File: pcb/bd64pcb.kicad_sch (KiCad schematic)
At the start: 225 parts, among them J1 USB_C_Receptacle_USB2.0, SW1 SW_Push, U1 ATmega32U4-MU, U2 IS31FL3733-QF, Y1 16MHz

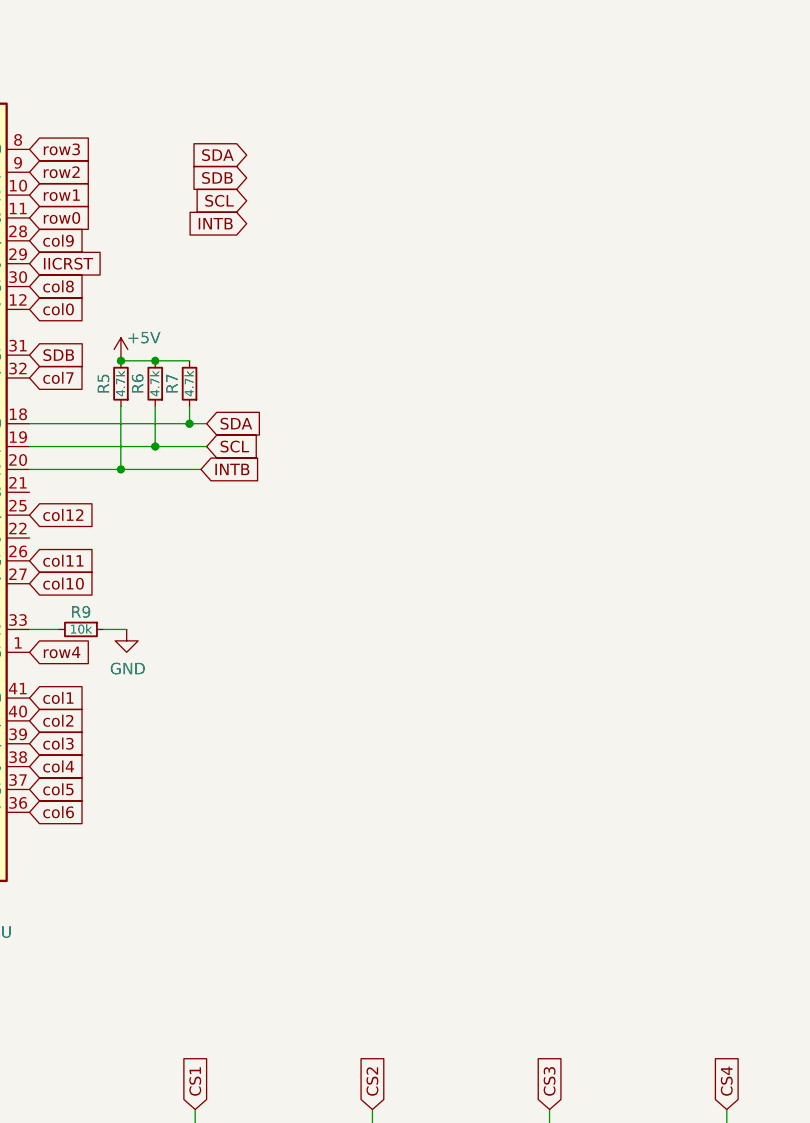
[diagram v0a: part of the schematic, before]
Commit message: reorg
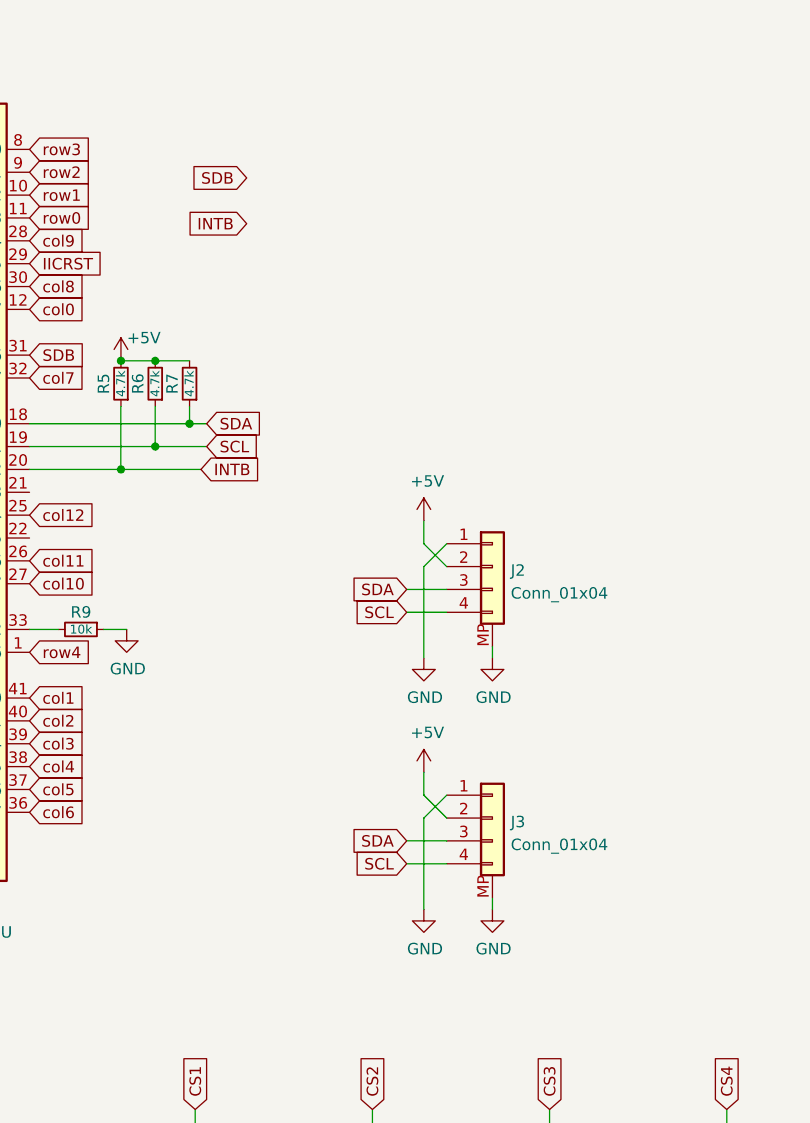
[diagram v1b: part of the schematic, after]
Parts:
- added J2, J3: Conn_01x04, Connector_JST:JST_SUR_SM04B-SURS-TF_1x04-1MP_P0.80mm_Horizontal, symbol Connector_Generic:Conn_01x04
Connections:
- net +5V: now also J2.2 (Pin_2), J3.2 (Pin_2)
- net GND: now also J2.1 (Pin_1), J2.MP, J3.1 (Pin_1), J3.MP
- net SCL: now also J2.4 (Pin_4), J3.4 (Pin_4)
- net SDA: now also J2.3 (Pin_3), J3.3 (Pin_3)
